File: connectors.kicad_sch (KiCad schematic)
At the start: 6 parts, among them J1 USB_C_Receptacle_USB2.0, J2 USB_C_Receptacle_USB2.0, J3 Screw_Terminal_01x02, J4 USB_A, U3 SRV05-4, U4 SRV05-4

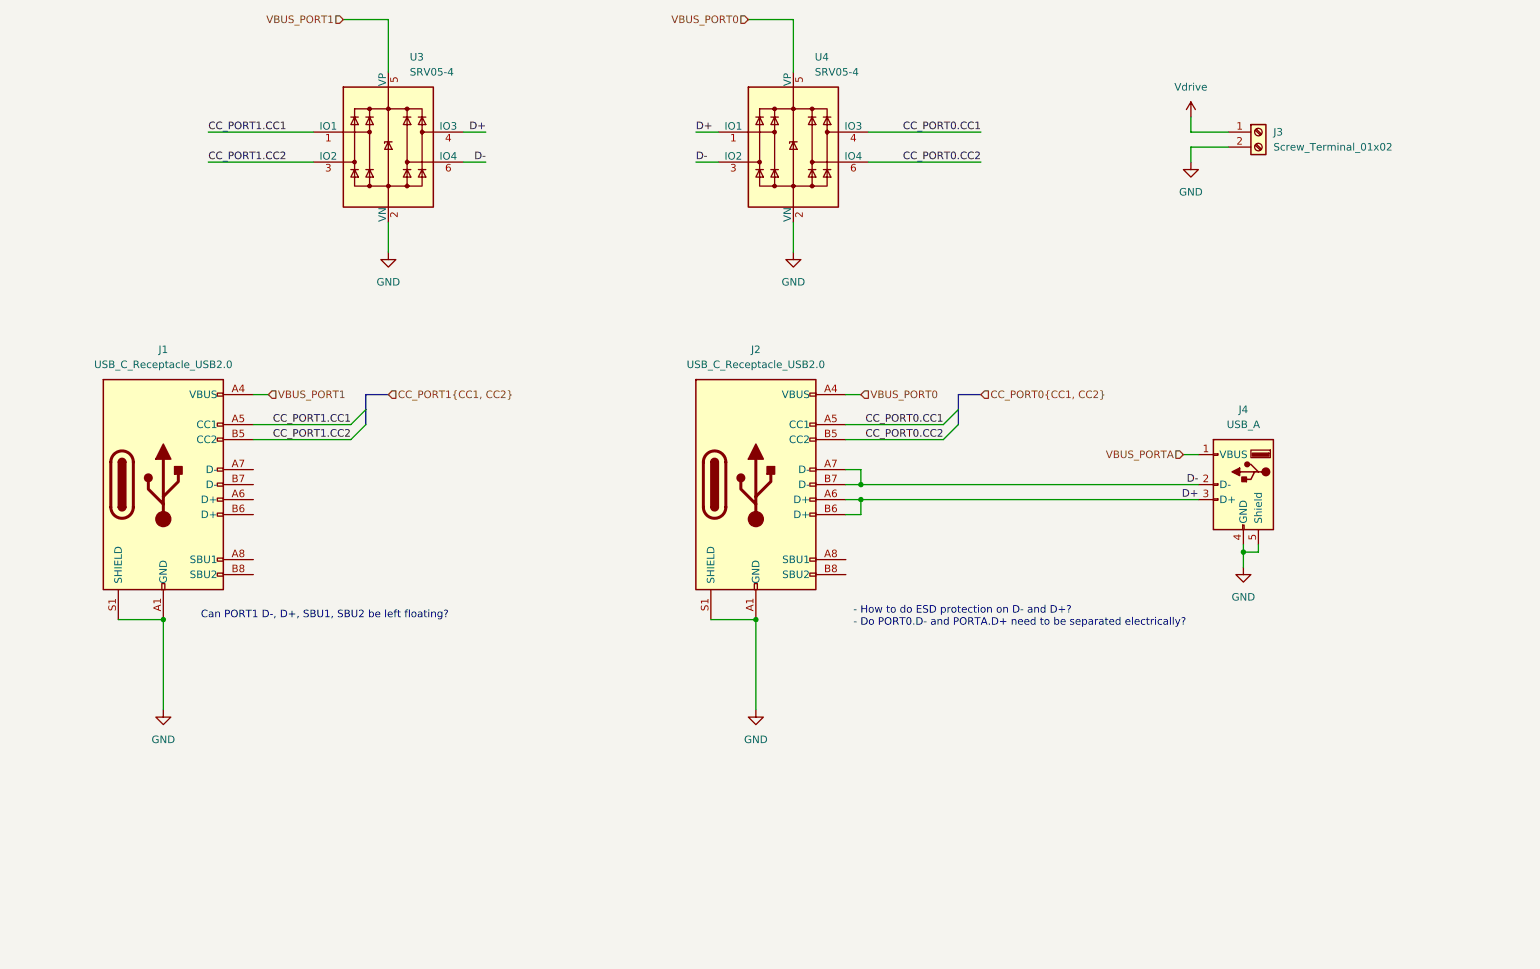
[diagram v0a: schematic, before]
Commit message: Wire more stuff
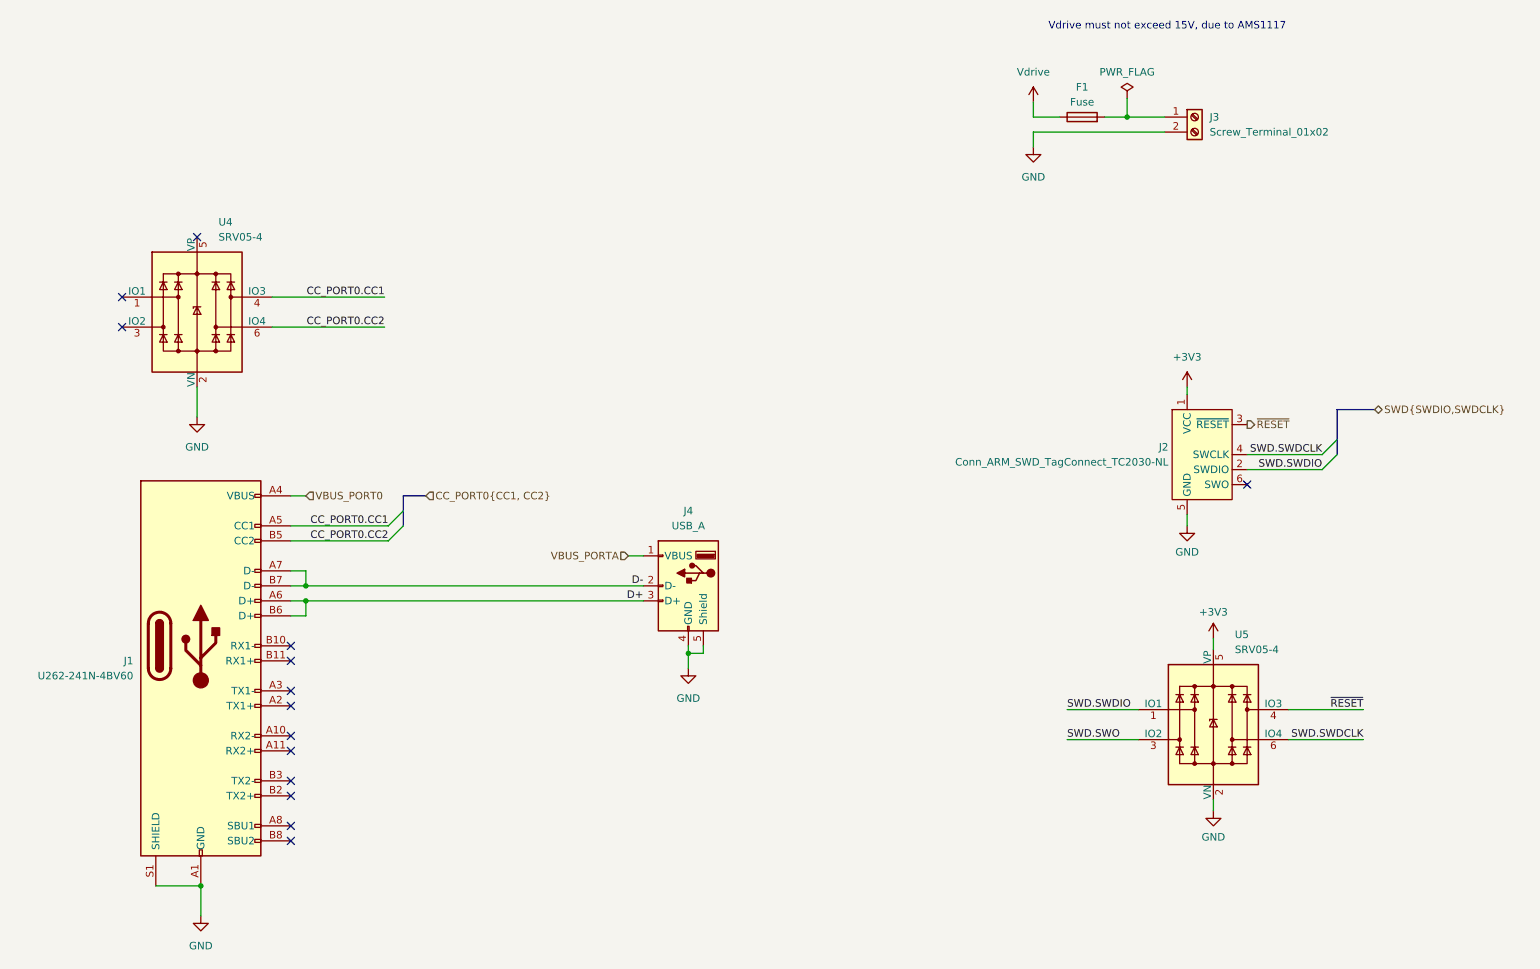
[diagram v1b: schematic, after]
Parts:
- removed J1, J2: USB_C_Receptacle_USB2.0, Connector_USB:USB_C_Receptacle_G-Switch_GT-USB-7010ASV, symbol Connector:USB_C_Receptacle_USB2.0
- removed U3: SRV05-4, Package_TO_SOT_SMD:SOT-23-6, symbol Power_Protection:SRV05-4
- added F1: Fuse, symbol Device:Fuse
- added J1: U262-241N-4BV60, Connector_USB:USB_C_Receptacle_Amphenol_12401548E4-2A, symbol Connector:USB_C_Receptacle
- added J2: Conn_ARM_SWD_TagConnect_TC2030-NL, Connector:Tag-Connect_TC2030-IDC-NL_2x03_P1.27mm_Vertical, symbol Connector:Conn_ARM_SWD_TagConnect_TC2030-NL
- added U5: SRV05-4, Package_TO_SOT_SMD:SOT-23-6, symbol Power_Protection:SRV05-4
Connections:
- net CC_PORT0.CC1: now also J1.A5 (CC1)
- net CC_PORT0.CC2: now also J1.B5 (CC2)
- net D+: now also J1.A6 (D+), J1.B6 (D+); no longer U4.1 (IO1)
- net D-: now also J1.A7 (D-), J1.B7 (D-); no longer U4.3 (IO2)
- net GND: now also J1.A1 (GND), J1.A12 (GND), J1.B1 (GND), J1.B12 (GND), J1.S1 (SHIELD), J2.5 (GND), U5.2 (VN)
- net VBUS_PORT0: now also J1.A4 (VBUS), J1.A9 (VBUS), J1.B4 (VBUS), J1.B9 (VBUS); no longer U4.5 (VP)
- net Vdrive: now also F1.1; no longer J3.1 (Pin_1)
- new net: F1.2, J3.1 (Pin_1)
- new net +3V3: J2.1 (VCC), U5.5 (VP)
- new net SWD.SWDCLK: J2.4 (SWCLK), U5.6 (IO4)
- new net SWD.SWDIO: J2.2 (SWDIO), U5.1 (IO1)
- new net SWD.SWO: U5.3 (IO2)
- new net ~{RESET}: J2.3 (~{RESET}), U5.4 (IO3)
- no-connect marks 0 -> 14
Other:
- note added: "Vdrive must not exceed 15V, due to AMS1117"
- note removed: "- How to do ESD protection on D- and D+? - Do PORT0.D- and PORTA.D+ need to be separated electrically?"
- note removed: "Can PORT1 D-, D+, SBU1, SBU2 be left floating?"
- moved on the sheet: J3, J4, U4

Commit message: Whole bunch of changes to all kinds of things
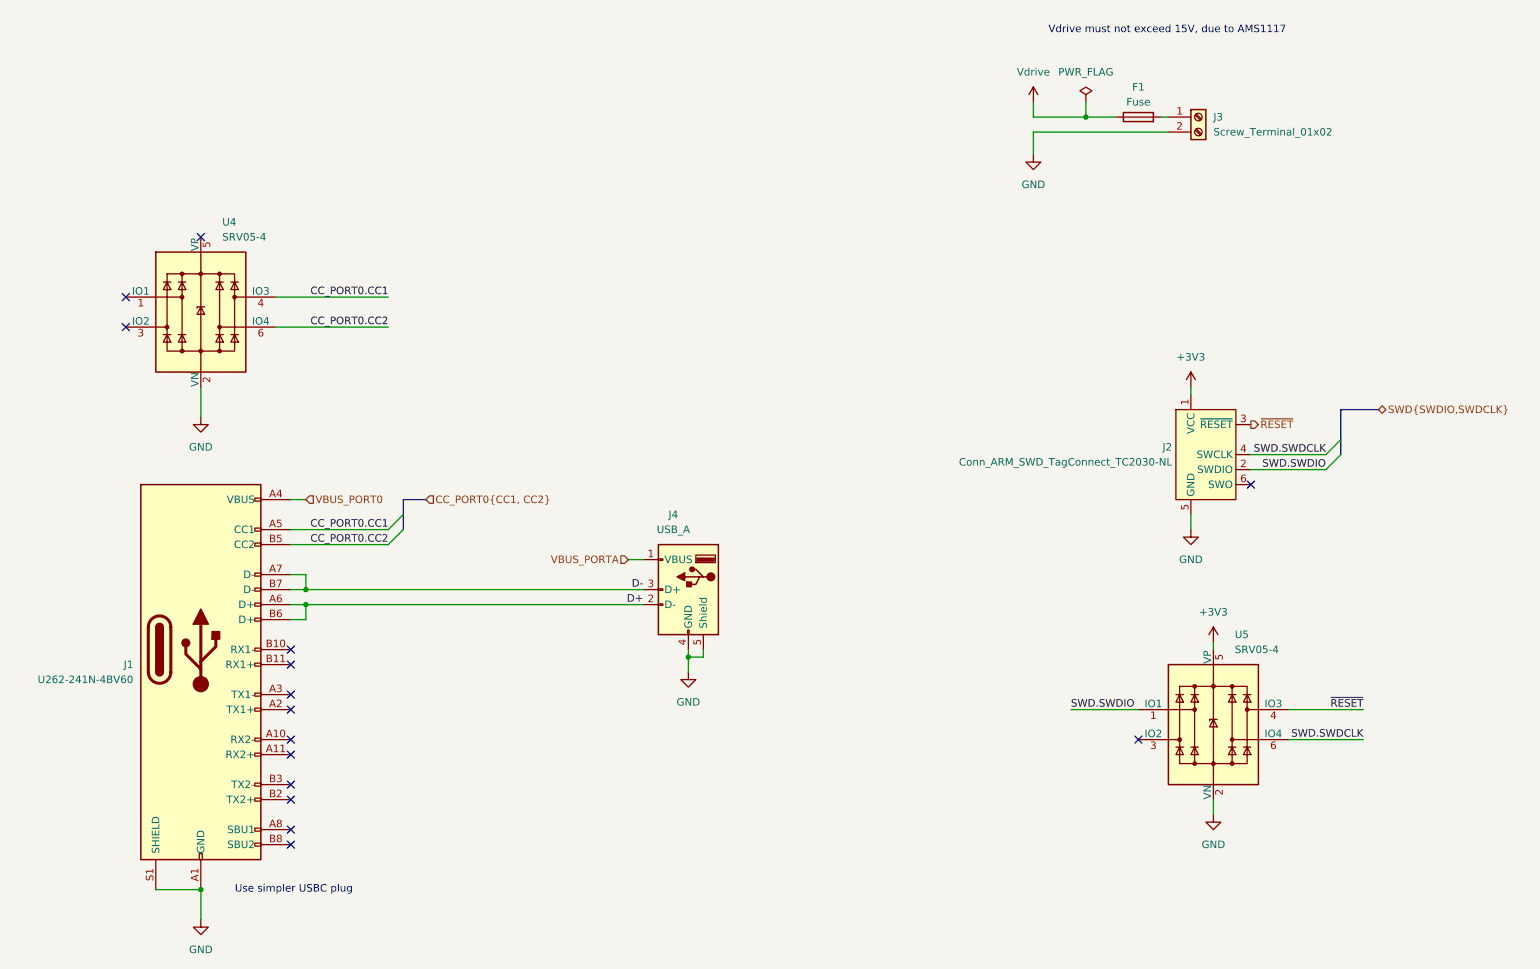
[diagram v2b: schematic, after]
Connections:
- net D+: now also J4.2 (D-); no longer J4.3 (D+)
- net D-: now also J4.3 (D+); no longer J4.2 (D-)
- net SWD.SWO: no longer names the net of U5.3 (IO2)
- no-connect marks 14 -> 15
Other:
- note added: "Use simpler USBC plug"
- moved on the sheet: F1, J1, J2, J3, J4, U4
